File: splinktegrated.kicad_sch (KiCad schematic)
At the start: 158 parts, among them J1 USB_C_Receptacle_USB2.0, J10 NA_Ribbon, J13 Conn_01x01_Socket, J14 Cirque, J15 Conn_01x01_Socket, J16 Conn_01x01_Socket, J17 Conn_01x01_Socket, J18 USB_C_Receptacle_USB2.0, J19 Conn_01x01_Socket, J20 Conn_01x01_Socket, J5 Conn_01x02, J7 NA_trackball, J8 NA_Ribbon, J9 NA_RGB, Q4 AO3401A, Q5 AO3401A, SW2 NA_SW_SPST, SW9001 NA_SW_SPST, U1 RP2040, U2 USBLC6-2P6, U3 XC6210B332MR-G, U4 USBLC6-2P6, U5 W25Q128JVS, U6 74LVC1T45, Y1 Crystal_GND24

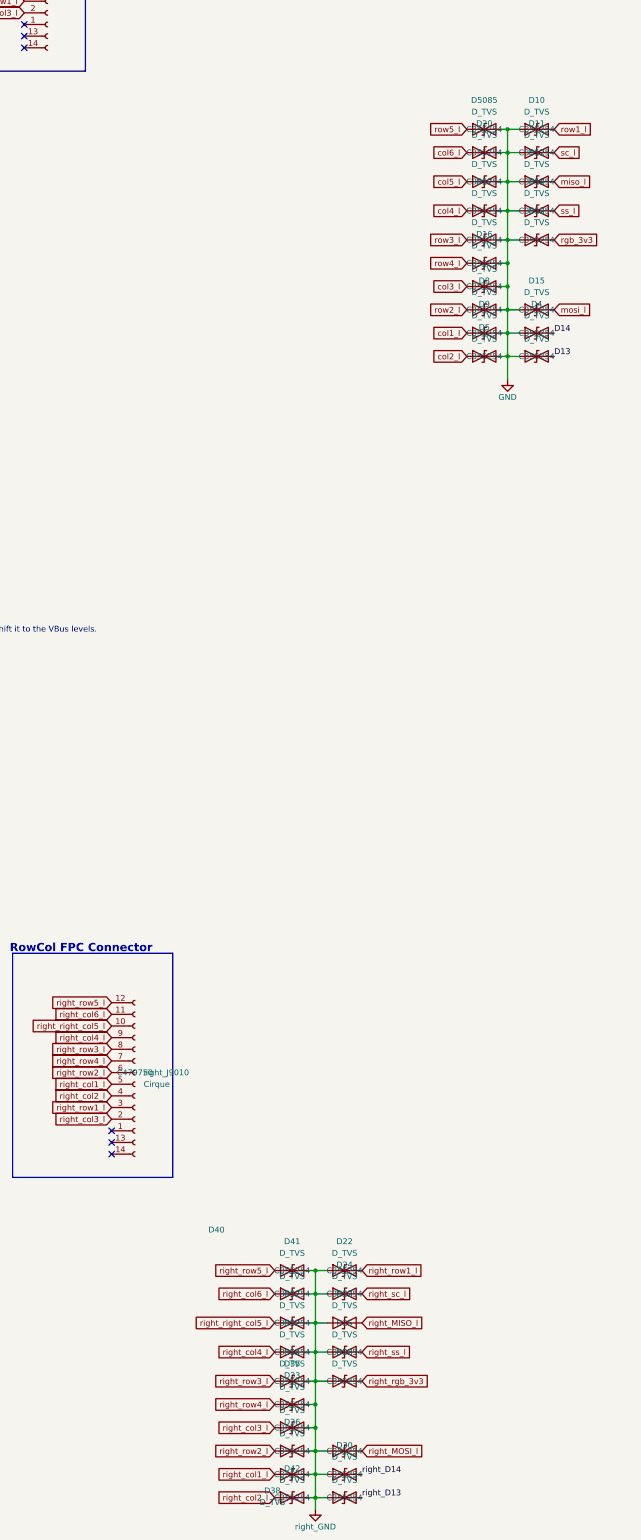
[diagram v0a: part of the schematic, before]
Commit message: silkscreen
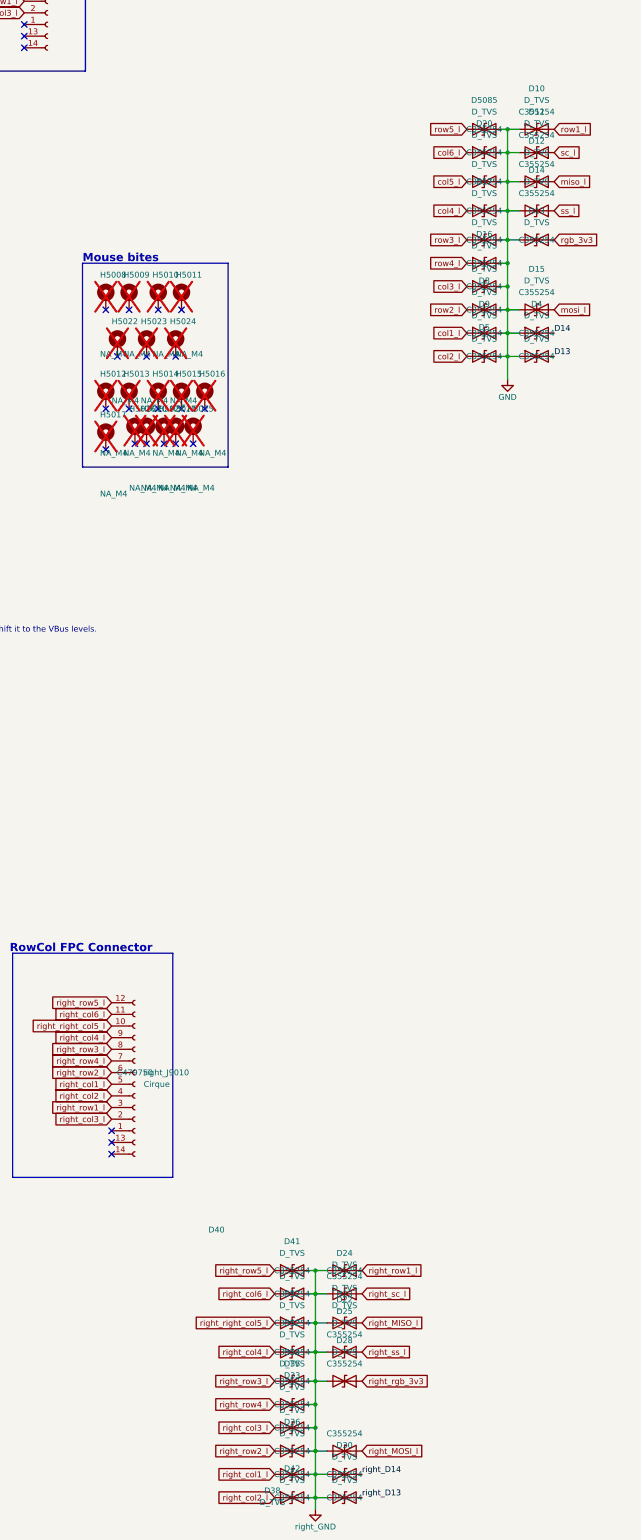
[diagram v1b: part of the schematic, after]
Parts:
- added H5008, H5009, H5010, H5011, H5012, H5013, H5014, H5015: NA_M4, local-libraries:mousebite, symbol Mechanical:MountingHole_Pad
- added H5016, H5017, H5020, H5021, H5022, H5023, H5024, H5025, H5026, H5027: NA_M4, local-libraries:mousebite_small, symbol Mechanical:MountingHole_Pad
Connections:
- net GND: now also D10.2 (A2), D11.2 (A2), D12.2 (A2), D14.2 (A2), D15.2 (A2); no longer D10.1 (A1), D11.1 (A1), D12.1 (A1), D14.1 (A1), D15.1 (A1)
- net miso_l: now also D12.1 (A1); no longer D12.2 (A2)
- net mosi_l: now also D15.1 (A1); no longer D15.2 (A2)
- net right_GND: now also D22.2 (A2), D23.2 (A2), D24.2 (A2), D25.2 (A2), D28.2 (A2), D29.2 (A2); no longer D22.1 (A1), D23.1 (A1), D24.1 (A1), D25.1 (A1), D28.1 (A1), D29.1 (A1)
- net right_MISO_l: now also D23.1 (A1); no longer D23.2 (A2)
- net right_MOSI_l: now also D29.1 (A1); no longer D29.2 (A2)
- net right_rgb_3v3: now also D28.1 (A1); no longer D28.2 (A2)
- net right_row1_l: now also D22.1 (A1); no longer D22.2 (A2)
- net right_sc_l: now also D24.1 (A1); no longer D24.2 (A2)
- net right_ss_l: now also D25.1 (A1); no longer D25.2 (A2)
- net row1_l: now also D10.1 (A1); no longer D10.2 (A2)
- net sc_l: now also D11.1 (A1); no longer D11.2 (A2)
- net ss_l: now also D14.1 (A1); no longer D14.2 (A2)
- no-connect marks 28 -> 46
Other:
- note added: "Mouse bites"
- moved on the sheet: D10, D11, D12, D14, D15, D22, D23, D24, D25, D28
